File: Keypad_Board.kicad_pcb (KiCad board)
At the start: 2 copper layers, 45 x 61 mm, 40 parts, among them IC1 STM32L010K4T6, IC2 TMUX136RSER, J3 Data_Conn, J4 SEL Jumper, J5 SW_Header, J6 BOOT Jumper

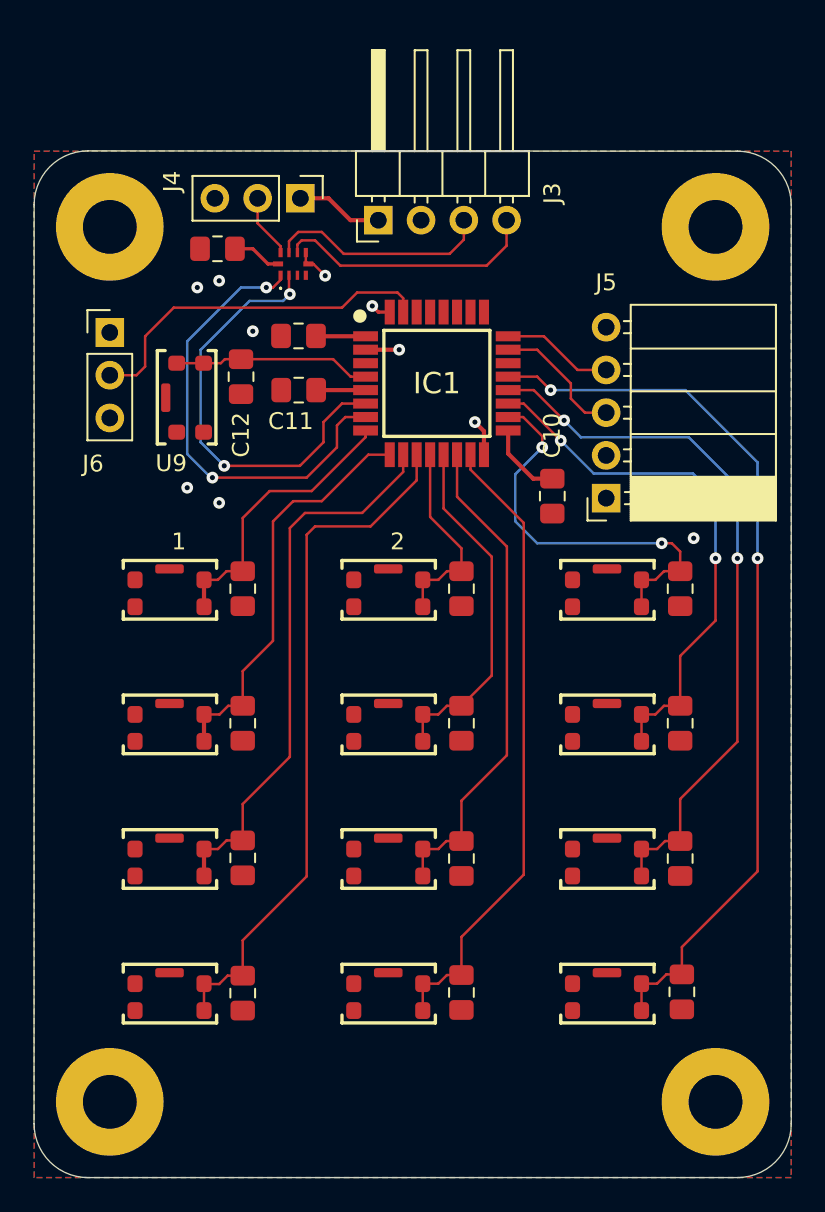
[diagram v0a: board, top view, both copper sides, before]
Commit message: update
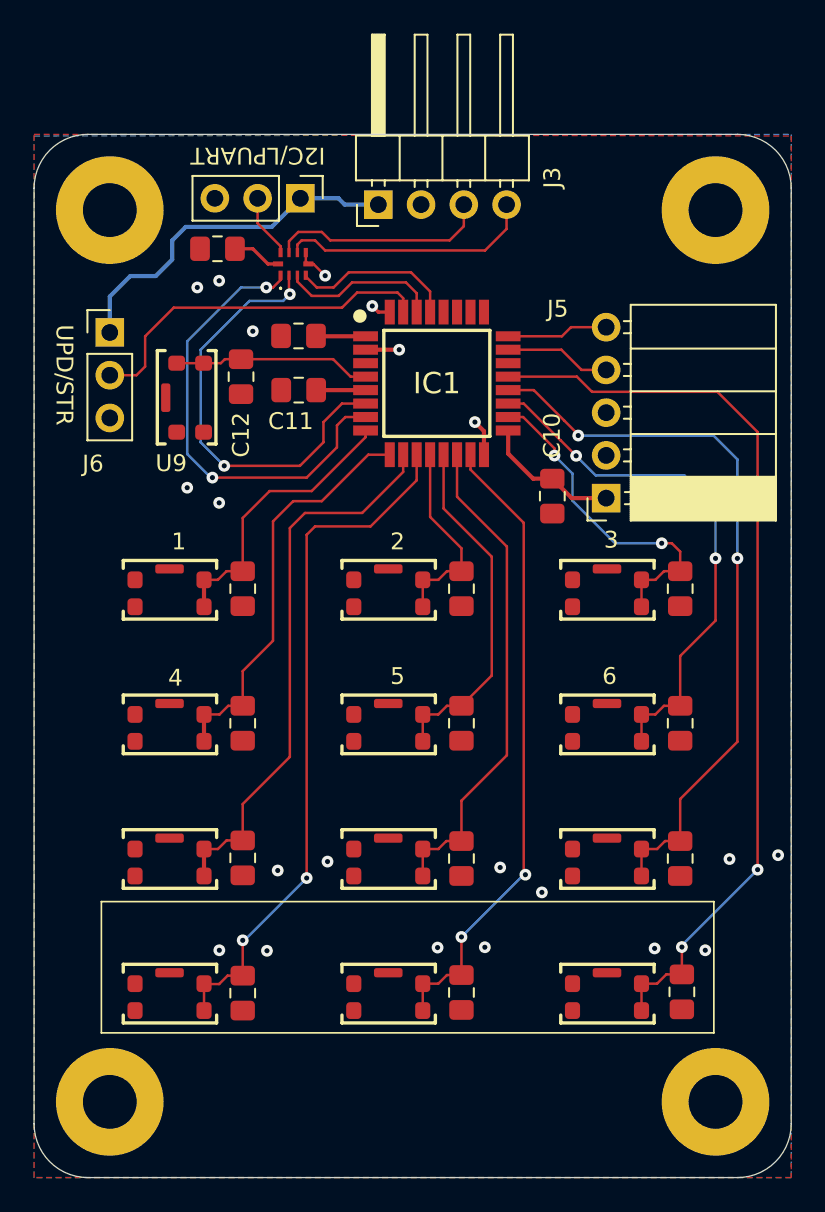
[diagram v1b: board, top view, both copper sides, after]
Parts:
- moved H1 1.00 mm to (114.5, 53.5)
- moved H2 1.00 mm to (150.5, 53.5)
- moved J3 0.93 mm to (130.5, 53.2)
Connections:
- J5 pad 3: /SYS_SWDIO -> /NRST
- J5 pad 4: /SYS_SWCLK -> /SYS_SWDIO
- J5 pad 5: /NRST -> /SYS_SWCLK
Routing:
- net +3.3V: track 18.6 -> 38.5 mm
- net /I2C1_SCL: track 0.00 -> 9.80 mm
- net /I2C1_SDA: track 0.00 -> 9.53 mm
- net /PA8: track 24.0 -> 20.0 mm
- net /SYS_SWDIO: track 7.90 -> 6.32 mm
- net /PA11: track 53.5 -> 54.5 mm
- net /PA10: track 42.6 -> 43.6 mm
- net /SYS_SWCLK: track 6.65 -> 6.05 mm
- net /PB1: track 37.9 -> 38.1 mm, vias 0 -> 2
- net /PA5: track 41.3 -> 41.4 mm, vias 0 -> 2
- net GND: vias 10 -> 21
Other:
- board size 45 x 61 mm -> 45 x 62 mm
- board text added: "3"
- board text added: "4"
- board text added: "5"
- board text added: "6"
- board text added: "I2C/LPUART"
- board text added: "UPD/STR"
